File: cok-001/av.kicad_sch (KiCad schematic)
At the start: 41 parts, among them Q2401 DTC144E, Q2402 SI2303BDS, U2402 MC78M09, U2403 MC78M05

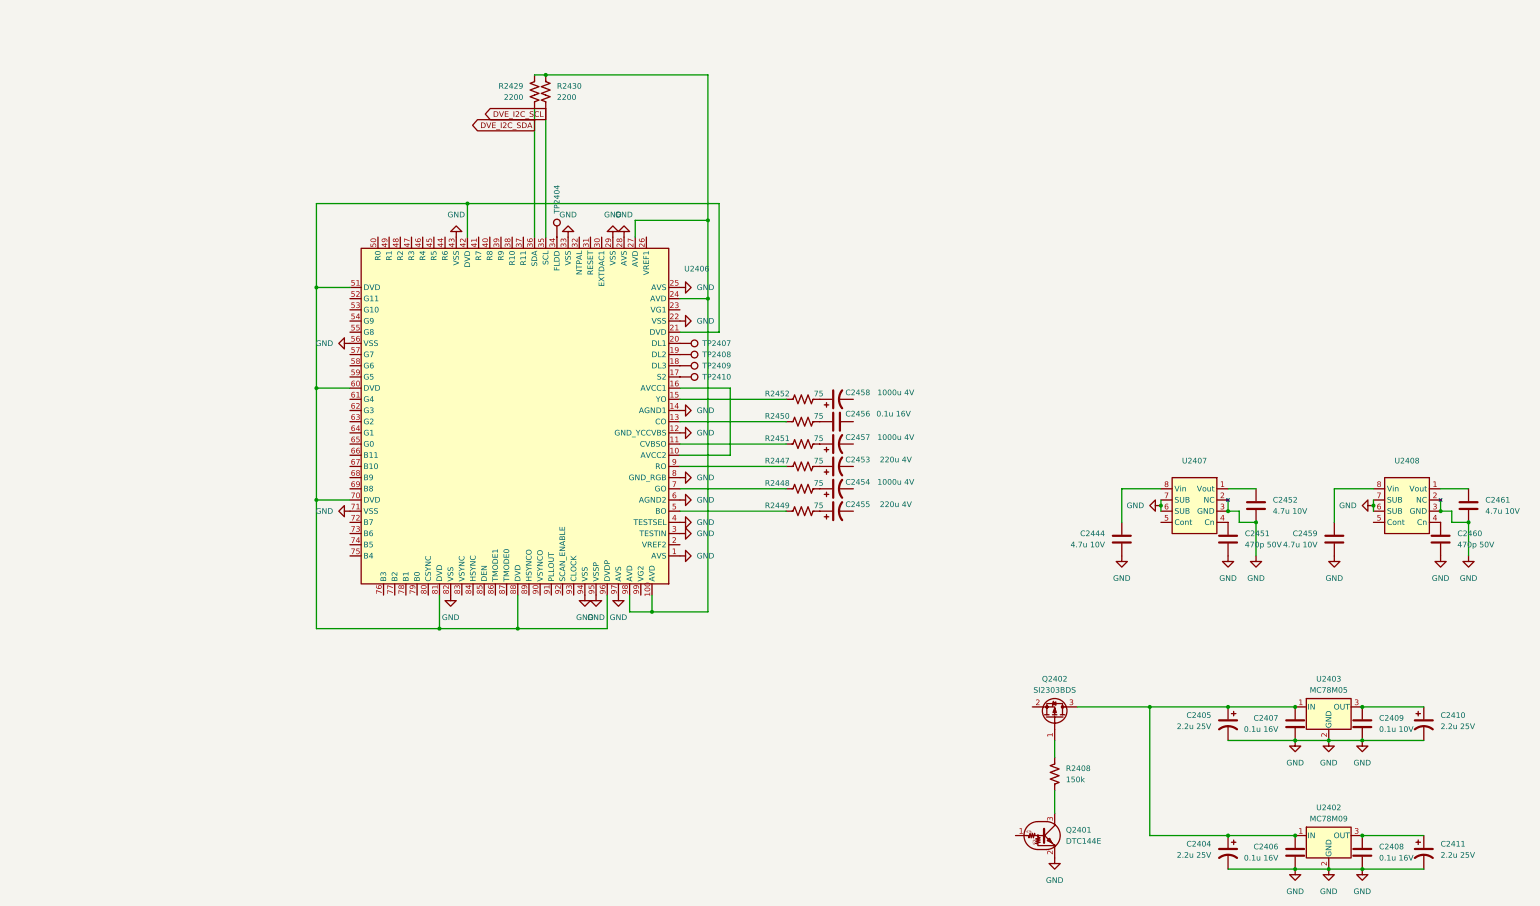
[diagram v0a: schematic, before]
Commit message: update to 9
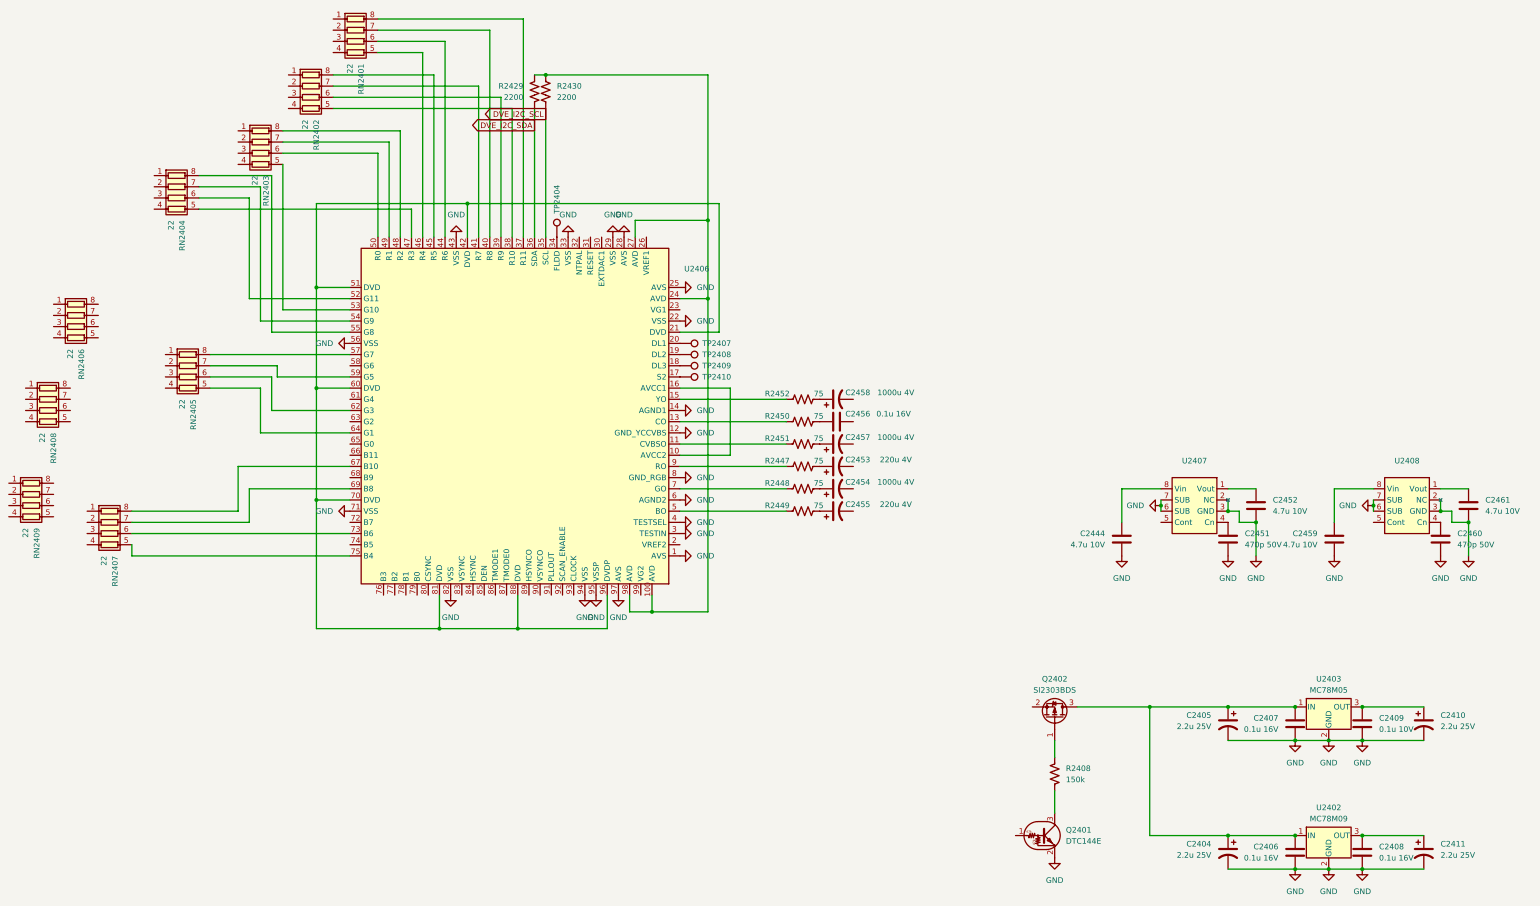
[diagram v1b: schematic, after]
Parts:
- added RN2401, RN2402, RN2403, RN2404, RN2405, RN2406, RN2407, RN2408, RN2409: 22, Resistor_SMD:R_Array_Convex_4x0402, symbol Device:R_Pack04
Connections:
- net at U2406.37 (R11): now also RN2401.8 (R1.2)
- net at U2406.38 (R10): now also RN2402.5 (R4.2)
- net at U2406.39 (R9): now also RN2402.6 (R3.2)
- net at U2406.40 (R8): now also RN2401.7 (R2.2)
- net at U2406.41 (R7): now also RN2402.7 (R2.2)
- net at U2406.44 (R6): now also RN2401.6 (R3.2)
- net at U2406.45 (R5): now also RN2402.8 (R1.2)
- net at U2406.46 (R4): now also RN2401.5 (R4.2)
- net at U2406.47 (R3): now also RN2404.5 (R4.2)
- net at U2406.48 (R2): now also RN2403.8 (R1.2)
- net at U2406.49 (R1): now also RN2403.7 (R2.2)
- net at U2406.50 (R0): now also RN2403.6 (R3.2)
- net at U2406.52 (G11): now also RN2404.6 (R3.2)
- net at U2406.53 (G10): now also RN2403.5 (R4.2)
- net at U2406.54 (G9): now also RN2404.7 (R2.2)
- net at U2406.55 (G8): now also RN2404.8 (R1.2)
- net at U2406.57 (G7): now also RN2405.8 (R1.2)
- net at U2406.59 (G5): now also RN2405.7 (R2.2)
- net at U2406.62 (G3): now also RN2405.6 (R3.2)
- net at U2406.64 (G1): now also RN2405.5 (R4.2)
- net at U2406.67 (B10): now also RN2407.8 (R1.2)
- net at U2406.69 (B8): now also RN2407.7 (R2.2)
- net at U2406.73 (B6): now also RN2407.6 (R3.2)
- net at U2406.75 (B4): now also RN2407.5 (R4.2)

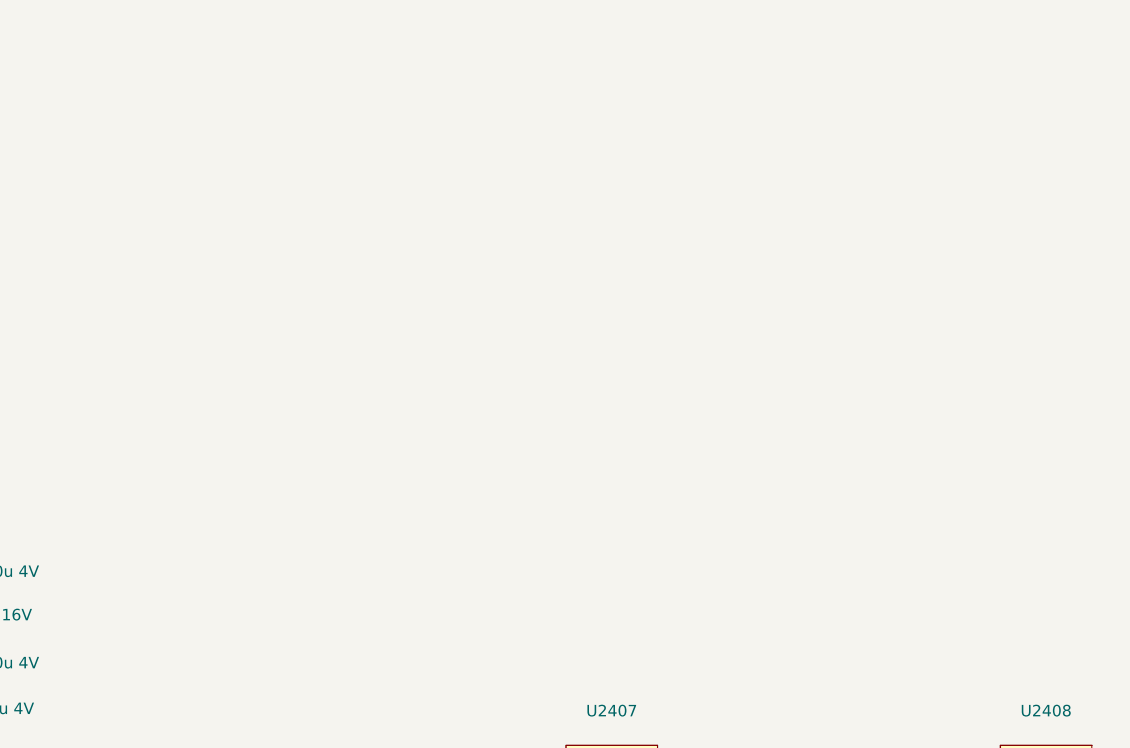
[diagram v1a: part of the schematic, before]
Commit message: footprints
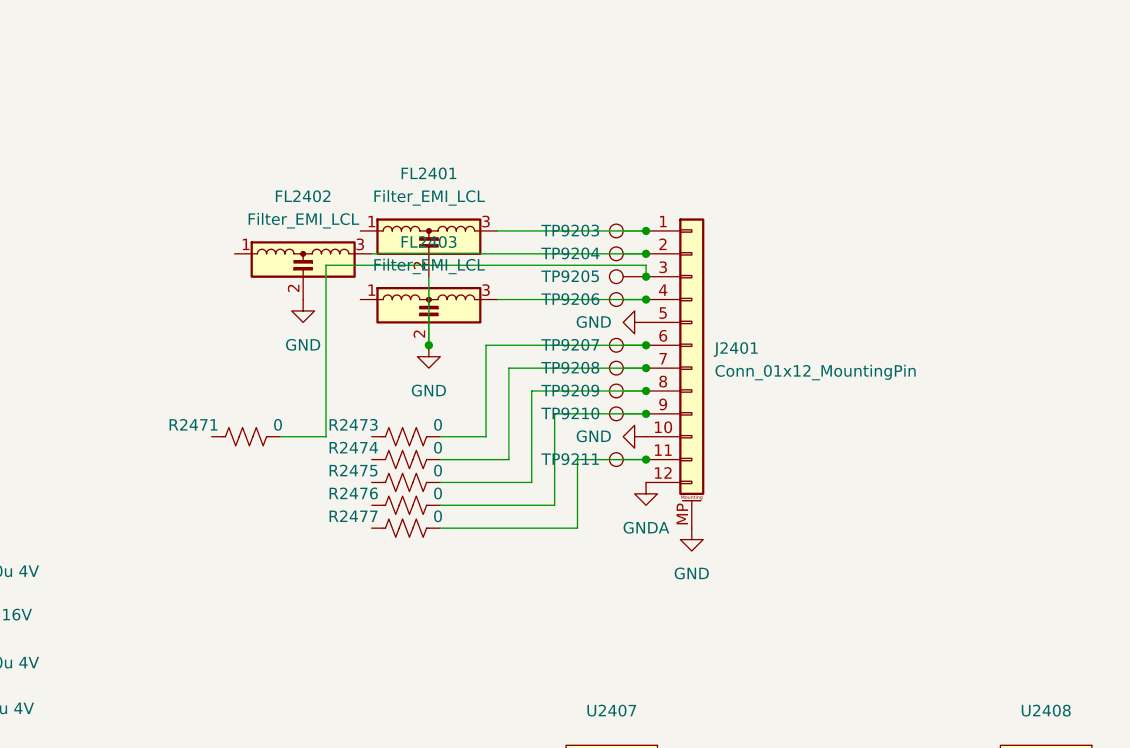
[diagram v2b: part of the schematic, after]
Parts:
- added FL2401, FL2402, FL2403: Filter_EMI_LCL, Filter:Filter_Mini-Circuits_FV1206-7, symbol Device:Filter_EMI_LCL
- added J2401: Conn_01x12_MountingPin, PS3:AVOUT, symbol Connector_Generic_MountingPin:Conn_01x12_MountingPin
- added R2471, R2473, R2474, R2475, R2476, R2477: 0, Resistor_SMD:R_0603_1608Metric, symbol Device:R_US
- added TP9203, TP9204, TP9205, TP9206, TP9207, TP9208, TP9209, TP9210, TP9211: TestPoint, TestPoint:TestPoint_Pad_D1.5mm, symbol Connector:TestPoint
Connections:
- net GND: now also FL2401.2, FL2402.2, FL2403.2, J2401.10 (Pin_10), J2401.5 (Pin_5), J2401.MP (MountPin)
- new net: FL2403.3, J2401.4 (Pin_4), TP9206.1
- new net: J2401.6 (Pin_6), R2473.2, TP9207.1
- new net: FL2401.3, J2401.1 (Pin_1), TP9203.1
- new net: J2401.9 (Pin_9), R2476.2, TP9210.1
- new net: J2401.3 (Pin_3), R2471.2, TP9205.1
- new net: J2401.8 (Pin_8), R2475.2, TP9209.1
- new net: FL2402.3, J2401.2 (Pin_2), TP9204.1
- new net: J2401.11 (Pin_11), R2477.2, TP9211.1
- new net: J2401.7 (Pin_7), R2474.2, TP9208.1
- new net GNDA: J2401.12 (Pin_12)
